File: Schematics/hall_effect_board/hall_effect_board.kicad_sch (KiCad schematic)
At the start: 5 parts, among them J1 B04B-PASK, U1 TMAG5273A1QDBVT

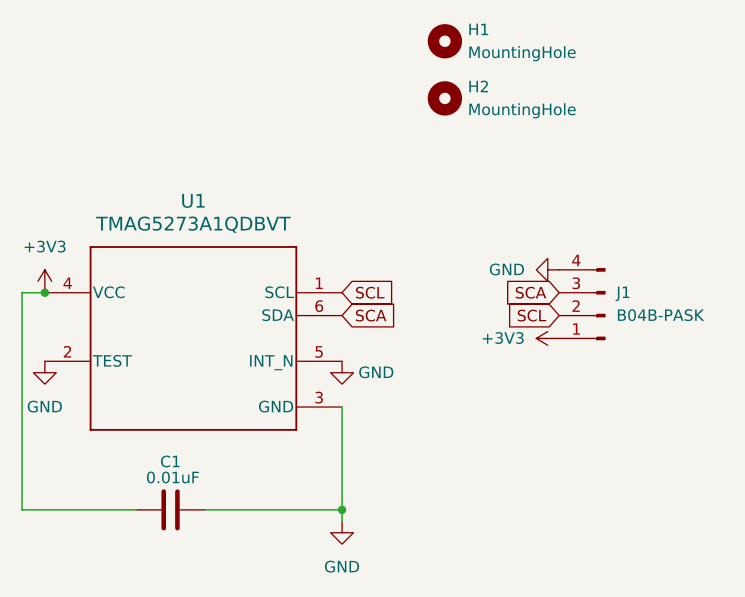
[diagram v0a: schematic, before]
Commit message: update for emily!!
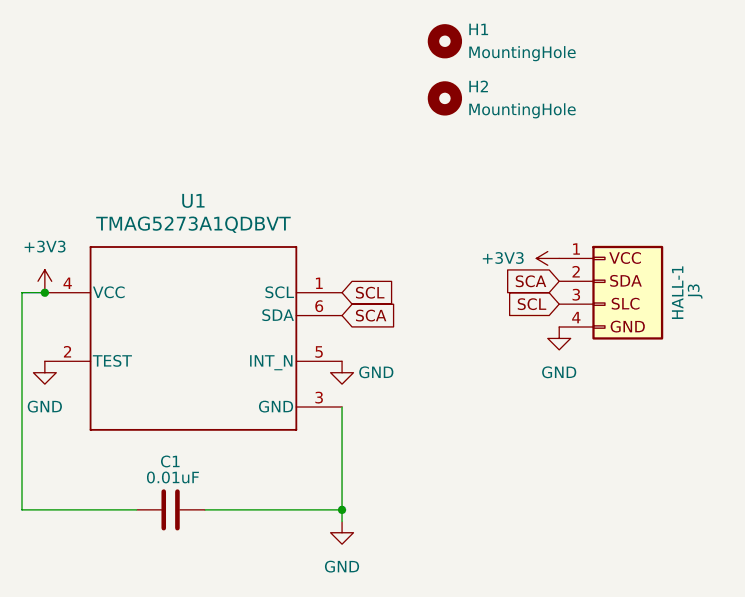
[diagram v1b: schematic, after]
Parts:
- removed J1: B04B-PASK, footprints:CONN_B04B-PASK_JST, symbol Connector:Conn_01x04_Pin
- added J3: HALL-1, footprints:CONN_SD-105309-100_04_MOL, symbol Connector_Generic:Conn_01x04
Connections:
- net +3V3: now also J3.1 (Pin_1)
- net GND: now also J3.4 (Pin_4)
- net SCA: now also J3.2 (Pin_2)
- net SCL: now also J3.3 (Pin_3)
